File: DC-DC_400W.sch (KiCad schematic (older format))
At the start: 13 parts, among them J1 Conn_01x24, J10 Conn_01x05, J2 Conn_01x03, J3 Conn_01x05, J4 Conn_01x01, J5 Conn_01x01, J6 Conn_01x02, J7 Conn_01x01, J8 Conn_01x01, J9 Conn_01x01

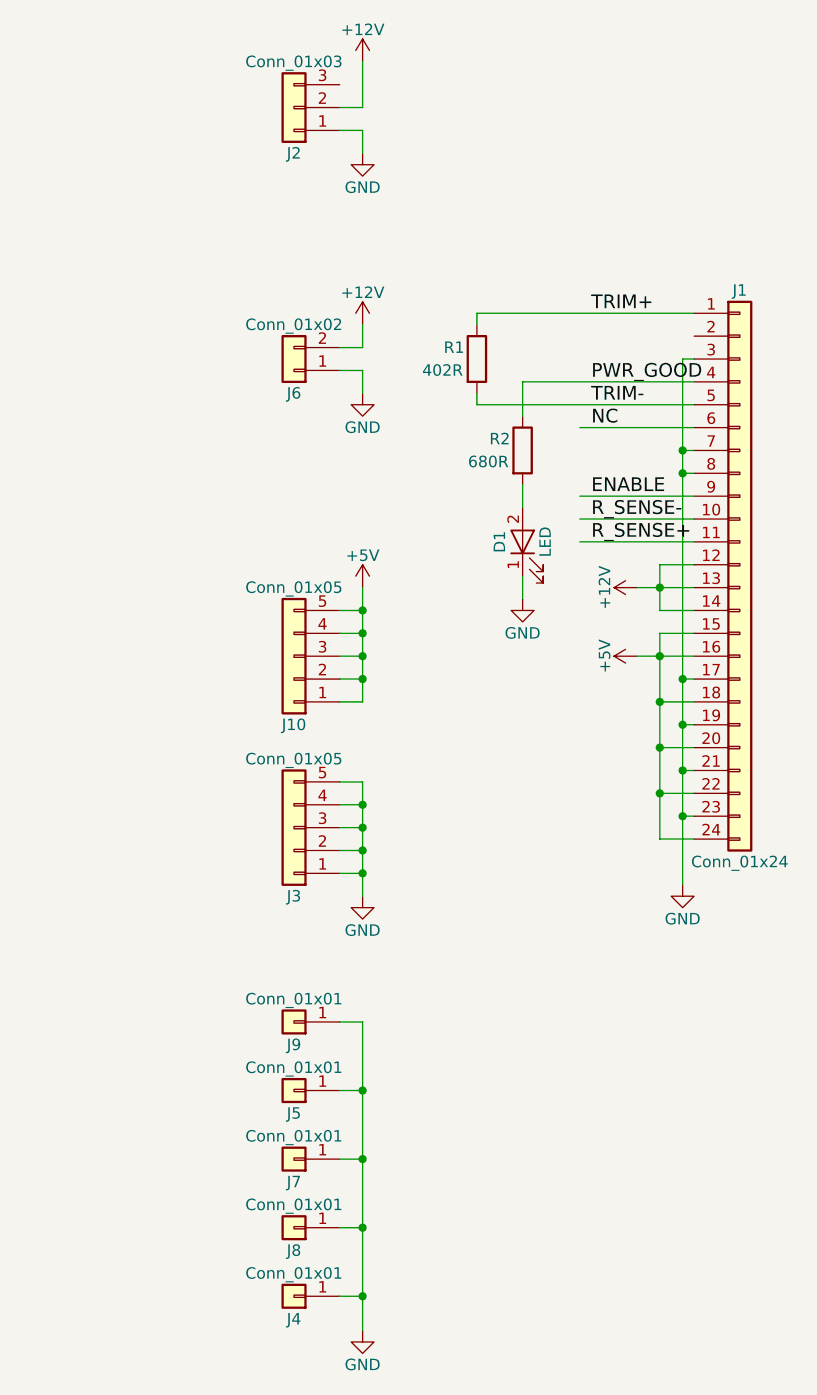
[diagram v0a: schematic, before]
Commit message: final 1.0 version
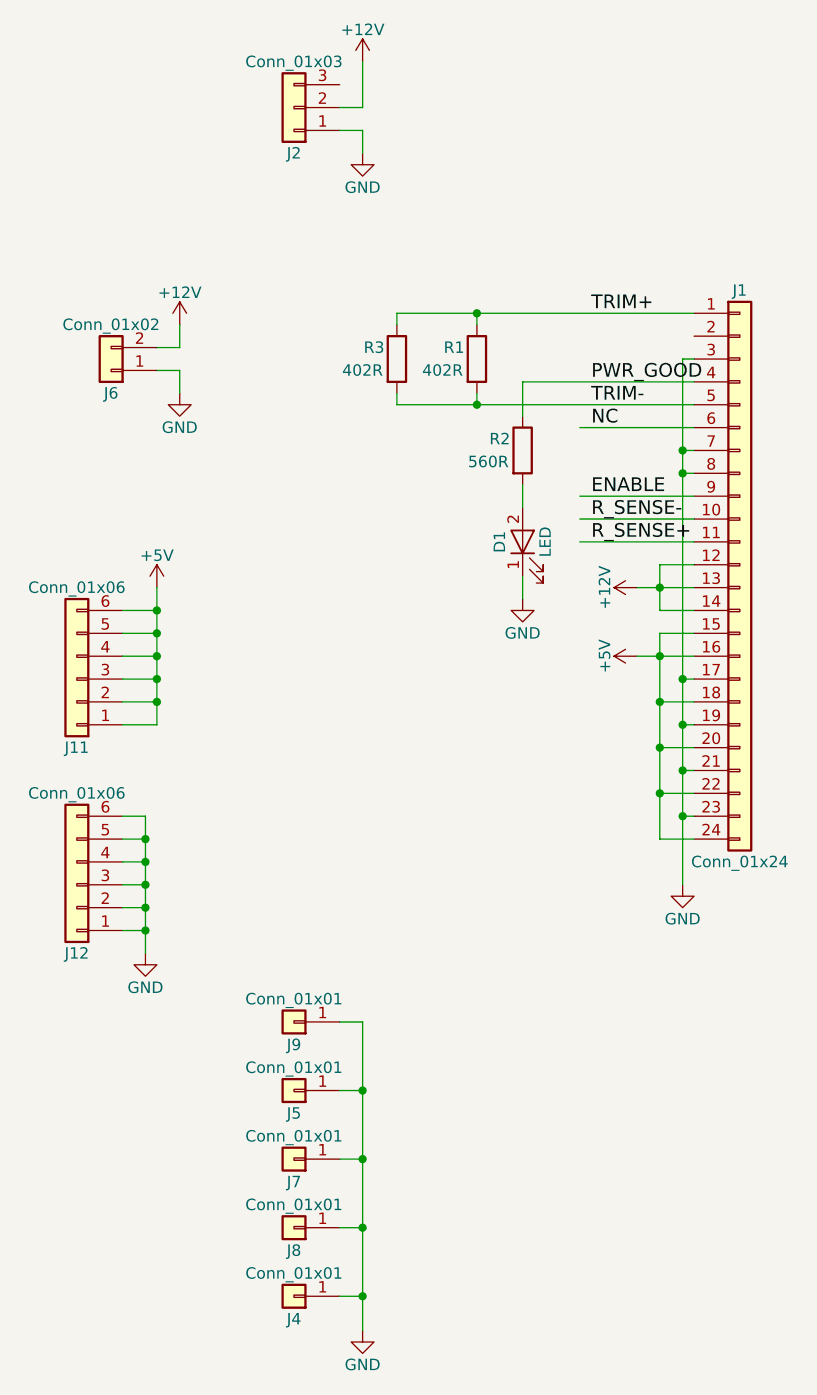
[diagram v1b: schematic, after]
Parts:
- removed J10, J3: Conn_01x05, Connectors_Phoenix:PhoenixContact_MSTBVA-G_05x5.00mm_Vertical, symbol Conn_01x05
- added J11, J12: Conn_01x06, Connectors_Phoenix:PhoenixContact_MSTBVA-G_06x5.00mm_Vertical, symbol Conn_01x06
- added R3: 402R, Resistors_SMD:R_0603, symbol R
- R2: value 680R -> 560R
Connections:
- wire segments 57 -> 61
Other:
- moved on the sheet: J6
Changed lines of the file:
@@
 $EndComp
 Wire Wire Line
-	5600 2150 6550 2150
+	5250 2150 6550 2150
 Wire Wire Line
 	5800 2450 6550 2450
 Wire Wire Line
-	5600 2550 6550 2550
+	5250 2550 6550 2550
 Wire Wire Line
 	6550 2650 6050 2650
@@
 	5600 2550 5600 2500
 $Comp
-L GND #PWR04
-U 1 1 5A3FEBAC
-P 5100 4700
-F 0 "#PWR04" H 5100 4450 50  0001 C CNN
-F 1 "GND" H 5100 4550 50  0000 C CNN
-F 2 "" H 5100 4700 50  0001 C CNN
-F 3 "" H 5100 4700 50  0001 C CNN
-	1    5100 4700
-	1    0    0    -1
-$EndComp
-Wire Wire Line
-	5100 4600 5000 4600
-Wire Wire Line
-	5100 4500 5000 4500
-Wire Wire Line
-	5100 4400 5000 4400
-Wire Wire Line
-	5000 4300 5100 4300
-Wire Wire Line
-	5000 4200 5100 4200
-$Comp
 L Conn_01x02 J6
 U 1 1 5A4F84EC
-P 4800 2400
-F 0 "J6" H 4800 2500 50  0000 C CNN
-F 1 "Conn_01x02" H 4800 2200 50  0000 C CNN
-F 2 "custom:XT60" H 4800 2400 50  0001 C CNN
-F 3 "" H 4800 2400 50  0001 C CNN
-	1    4800 2400
-	-1   0    0    1
-$EndComp
-$Comp
-L +12V #PWR05
+P 4000 2400
+F 0 "J6" H 4000 2500 50  0000 C CNN
+F 1 "Conn_01x02" H 4000 2200 50  0000 C CNN
+F 2 "custom:XT60" H 4000 2400 50  0001 C CNN
+F 3 "" H 4000 2400 50  0001 C CNN
+	1    4000 2400
+	-1   0    0    1
+$EndComp
+$Comp
+L +12V #PWR04
 U 1 1 5A4F85E8
-P 5100 2200
-F 0 "#PWR05" H 5100 2050 50  0001 C CNN
-F 1 "+12V" H 5100 2340 50  0000 C CNN
-F 2 "" H 5100 2200 50  0001 C CNN
-F 3 "" H 5100 2200 50  0001 C CNN
-	1    5100 2200
-	1    0    0    -1
-$EndComp
-$Comp
-L GND #PWR06
+P 4300 2200
+F 0 "#PWR04" H 4300 2050 50  0001 C CNN
+F 1 "+12V" H 4300 2340 50  0000 C CNN
+F 2 "" H 4300 2200 50  0001 C CNN
+F 3 "" H 4300 2200 50  0001 C CNN
+	1    4300 2200
+	1    0    0    -1
+$EndComp
+$Comp
+L GND #PWR05
 U 1 1 5A4F8A4D
-P 5100 2500
-F 0 "#PWR06" H 5100 2250 50  0001 C CNN
-F 1 "GND" H 5100 2350 50  0000 C CNN
-F 2 "" H 5100 2500 50  0001 C CNN
-F 3 "" H 5100 2500 50  0001 C CNN
-	1    5100 2500
-	1    0    0    -1
-$EndComp
-Wire Wire Line
-	5000 2300 5100 2300
-Wire Wire Line
-	5100 2300 5100 2200
-Wire Wire Line
-	5000 2400 5100 2400
-Wire Wire Line
-	5100 2400 5100 2500
+P 4300 2500
+F 0 "#PWR05" H 4300 2250 50  0001 C CNN
+F 1 "GND" H 4300 2350 50  0000 C CNN
+F 2 "" H 4300 2500 50  0001 C CNN
+F 3 "" H 4300 2500 50  0001 C CNN
+	1    4300 2500
+	1    0    0    -1
+$EndComp
+Wire Wire Line
+	4200 2300 4300 2300
+Wire Wire Line
+	4300 2300 4300 2200
+Wire Wire Line
+	4200 2400 4300 2400
+Wire Wire Line
+	4300 2400 4300 2500
 $Comp
 L Conn_01x03 J2
@@
 $EndComp
 $Comp
-L GND #PWR07
+L GND #PWR06
 U 1 1 5A58C603
 P 5100 1450
-F 0 "#PWR07" H 5100 1200 50  0001 C CNN
+F 0 "#PWR06" H 5100 1200 50  0001 C CNN
 F 1 "GND" H 5100 1300 50  0000 C CNN
 F 2 "" H 5100 1450 50  0001 C CNN
@@
 $EndComp
 $Comp
-L +12V #PWR08
+L +12V #PWR07
 U 1 1 5A58C626
 P 5100 1050
-F 0 "#PWR08" H 5100 900 50  0001 C CNN
+F 0 "#PWR07" H 5100 900 50  0001 C CNN
 F 1 "+12V" H 5100 1190 50  0000 C CNN
 F 2 "" H 5100 1050 50  0001 C CNN
@@
 P 5800 2750
 F 0 "R2" H 5700 2800 50  0000 C CNN
-F 1 "680R" H 5650 2700 50  0000 C CNN
+F 1 "560R" H 5650 2700 50  0000 C CNN
 F 2 "Resistors_SMD:R_0603" V 5730 2750 50  0001 C CNN
 F 3 "" H 5800 2750 50  0001 C CNN
@@
 $EndComp
 $Comp
-L GND #PWR09
+L GND #PWR08
 U 1 1 5A5A0040
 P 5800 3400
-F 0 "#PWR09" H 5800 3150 50  0001 C CNN
+F 0 "#PWR08" H 5800 3150 50  0001 C CNN
 F 1 "GND" H 5800 3250 50  0000 C CNN
 F 2 "" H 5800 3400 50  0001 C CNN
@@
 $EndComp
 $Comp
-L GND #PWR010
+L GND #PWR09
 U 1 1 5A5A623B
 P 5100 6600
-F 0 "#PWR010" H 5100 6350 50  0001 C CNN
+F 0 "#PWR09" H 5100 6350 50  0001 C CNN
 F 1 "GND" H 5100 6450 50  0000 C CNN
 F 2 "" H 5100 6600 50  0001 C CNN
@@
 Connection ~ 5100 5550
 $Comp
-L Conn_01x05 J10
-U 1 1 5A5C6ADB
-P 4800 3650
-F 0 "J10" H 4800 3950 50  0000 C CNN
-F 1 "Conn_01x05" H 4800 3350 50  0000 C CNN
-F 2 "Connectors_Phoenix:PhoenixContact_MSTBVA-G_05x5.00mm_Vertical" H 4800 3650 50  0001 C CNN
-F 3 "" H 4800 3650 50  0001 C CNN
-	1    4800 3650
-	-1   0    0    1
-$EndComp
-$Comp
-L +5V #PWR011
-U 1 1 5A5CBC89
-P 5100 3350
-F 0 "#PWR011" H 5100 3200 50  0001 C CNN
-F 1 "+5V" H 5100 3490 50  0000 C CNN
-F 2 "" H 5100 3350 50  0001 C CNN
-F 3 "" H 5100 3350 50  0001 C CNN
-	1    5100 3350
-	1    0    0    -1
-$EndComp
-Wire Wire Line
-	5100 3850 5000 3850
-Wire Wire Line
-	5100 3350 5100 3850
-Wire Wire Line
-	5000 3450 5100 3450
-Connection ~ 5100 3450
-Wire Wire Line
-	5000 3550 5100 3550
-Connection ~ 5100 3550
-Wire Wire Line
-	5000 3650 5100 3650
-Connection ~ 5100 3650
-Wire Wire Line
-	5000 3750 5100 3750
-Connection ~ 5100 3750
-$Comp
-L Conn_01x05 J3
-U 1 1 5A5CC2F8
-P 4800 4400
-F 0 "J3" H 4800 4700 50  0000 C CNN
-F 1 "Conn_01x05" H 4800 4100 50  0000 C CNN
-F 2 "Connectors_Phoenix:PhoenixContact_MSTBVA-G_05x5.00mm_Vertical" H 4800 4400 50  0001 C CNN
-F 3 "" H 4800 4400 50  0001 C CNN
-	1    4800 4400
-	-1   0    0    1
-$EndComp
-Wire Wire Line
-	5100 4200 5100 4700
-Connection ~ 5100 4600
-Connection ~ 5100 4500
-Connection ~ 5100 4400
-Connection ~ 5100 4300
-$Comp
 L Conn_01x01 J4
 U 1 1 5A5DC987
@@
 	5000 6450 5100 6450
 Connection ~ 5100 6450
+$Comp
+L R R3
+U 1 1 5A7EB192
+P 5250 2350
+F 0 "R3" H 5150 2400 50  0000 C CNN
+F 1 "402R" H 5100 2300 50  0000 C CNN
+F 2 "Resistors_SMD:R_0603" V 5180 2350 50  0001 C CNN
+F 3 "" H 5250 2350 50  0001 C CNN
+	1    5250 2350
+	1    0    0    -1
+$EndComp
+Wire Wire Line
+	5250 2200 5250 2150
+Connection ~ 5600 2150
+Wire Wire Line
+	5250 2500 5250 2550
+Connection ~ 5600 2550
+$Comp
+L Conn_01x06 J11
+U 1 1 5A7EB3AF
+P 3850 3750
+F 0 "J11" H 3850 4050 50  0000 C CNN
+F 1 "Conn_01x06" H 3850 3350 50  0000 C CNN
+F 2 "Connectors_Phoenix:PhoenixContact_MSTBVA-G_06x5.00mm_Vertical" H 3850 3750 50  0001 C CNN
+F 3 "" H 3850 3750 50  0001 C CNN
+	1    3850 3750
+	-1   0    0    1
+$EndComp
+$Comp
+L Conn_01x06 J12
+U 1 1 5A7EB42F
+P 3850 4650
+F 0 "J12" H 3850 4950 50  0000 C CNN
+F 1 "Conn_01x06" H 3850 4250 50  0000 C CNN
+F 2 "Connectors_Phoenix:PhoenixContact_MSTBVA-G_06x5.00mm_Vertical" H 3850 4650 50  0001 C CNN
+F 3 "" H 3850 4650 50  0001 C CNN
+	1    3850 4650
+	-1   0    0    1
+$EndComp
+$Comp
+L +5V #PWR010
+U 1 1 5A7EB553
+P 4200 3350
+F 0 "#PWR010" H 4200 3200 50  0001 C CNN
+F 1 "+5V" H 4200 3490 50  0000 C CNN
+F 2 "" H 4200 3350 50  0001 C CNN
+F 3 "" H 4200 3350 50  0001 C CNN
+	1    4200 3350
+	1    0    0    -1
+$EndComp
+Wire Wire Line
+	4050 3950 4200 3950
+Wire Wire Line
+	4200 3950 4200 3350
+Wire Wire Line
+	4050 3450 4200 3450
+Connection ~ 4200 3450
+Wire Wire Line
+	4050 3550 4200 3550
+Connection ~ 4200 3550
+Wire Wire Line
+	4050 3650 4200 3650
+Connection ~ 4200 3650
+Wire Wire Line
+	4050 3750 4200 3750
+Connection ~ 4200 3750
+Wire Wire Line
+	4050 3850 4200 3850
+Connection ~ 4200 3850
+$Comp
+L GND #PWR011
+U 1 1 5A7EB885
+P 4150 4950
+F 0 "#PWR011" H 4150 4700 50  0001 C CNN
+F 1 "GND" H 4150 4800 50  0000 C CNN
+F 2 "" H 4150 4950 50  0001 C CNN
+F 3 "" H 4150 4950 50  0001 C CNN
+	1    4150 4950
+	1    0    0    -1
+$EndComp
+Wire Wire Line
+	4050 4350 4150 4350
+Wire Wire Line
+	4150 4350 4150 4950
+Wire Wire Line
+	4050 4450 4150 4450
+Connection ~ 4150 4450
+Wire Wire Line
+	4050 4550 4150 4550
+Connection ~ 4150 4550
+Wire Wire Line
+	4050 4650 4150 4650
+Connection ~ 4150 4650
+Wire Wire Line
+	4050 4750 4150 4750
+Connection ~ 4150 4750
+Wire Wire Line
+	4050 4850 4150 4850
+Connection ~ 4150 4850
 $EndSCHEMATC
